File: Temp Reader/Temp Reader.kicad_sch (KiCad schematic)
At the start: 19 parts, among them U1 ESP32-WROOM-32, U2 BME280, U4 NRF24L01_Breakout, U5 AP62150WU

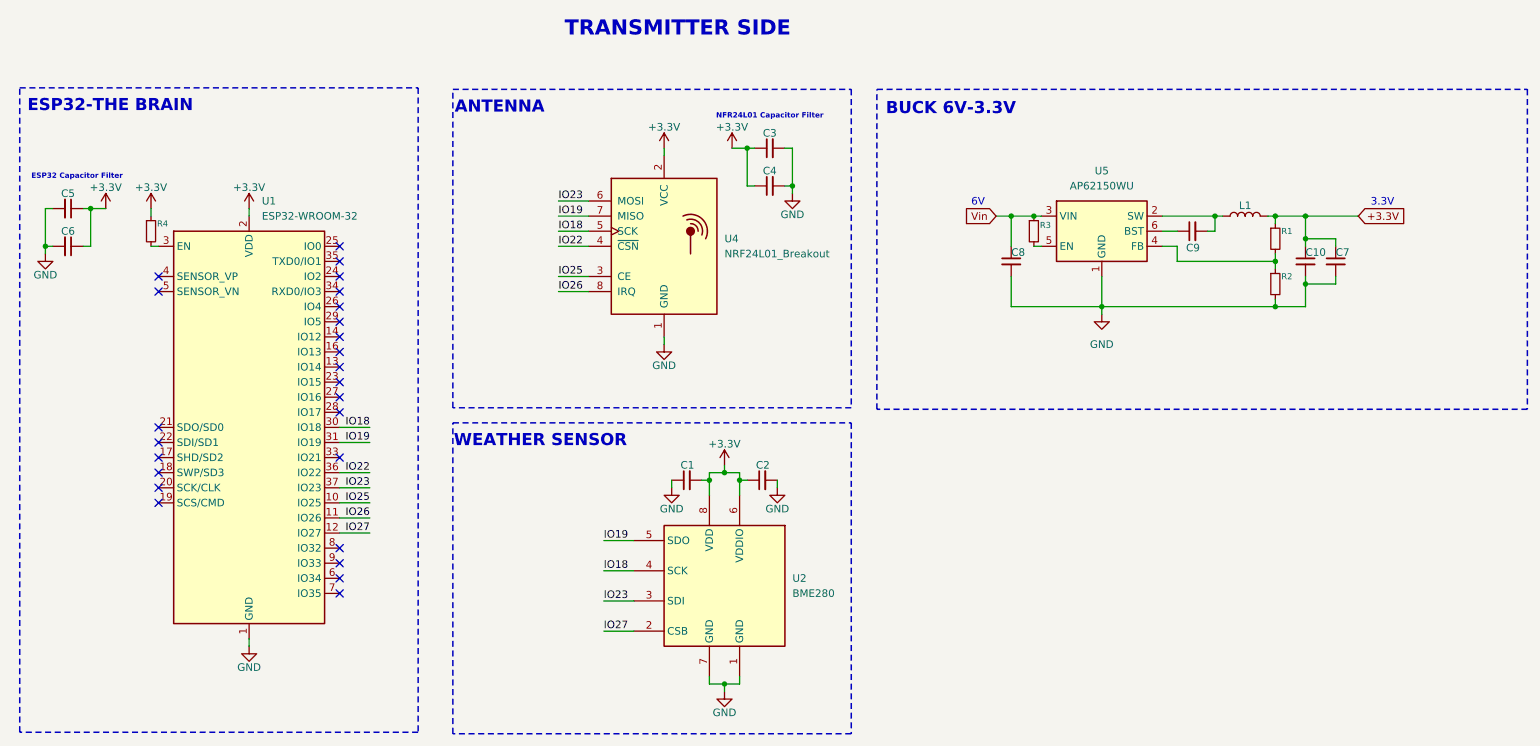
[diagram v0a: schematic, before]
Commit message: Final Schematic v 0.1.0
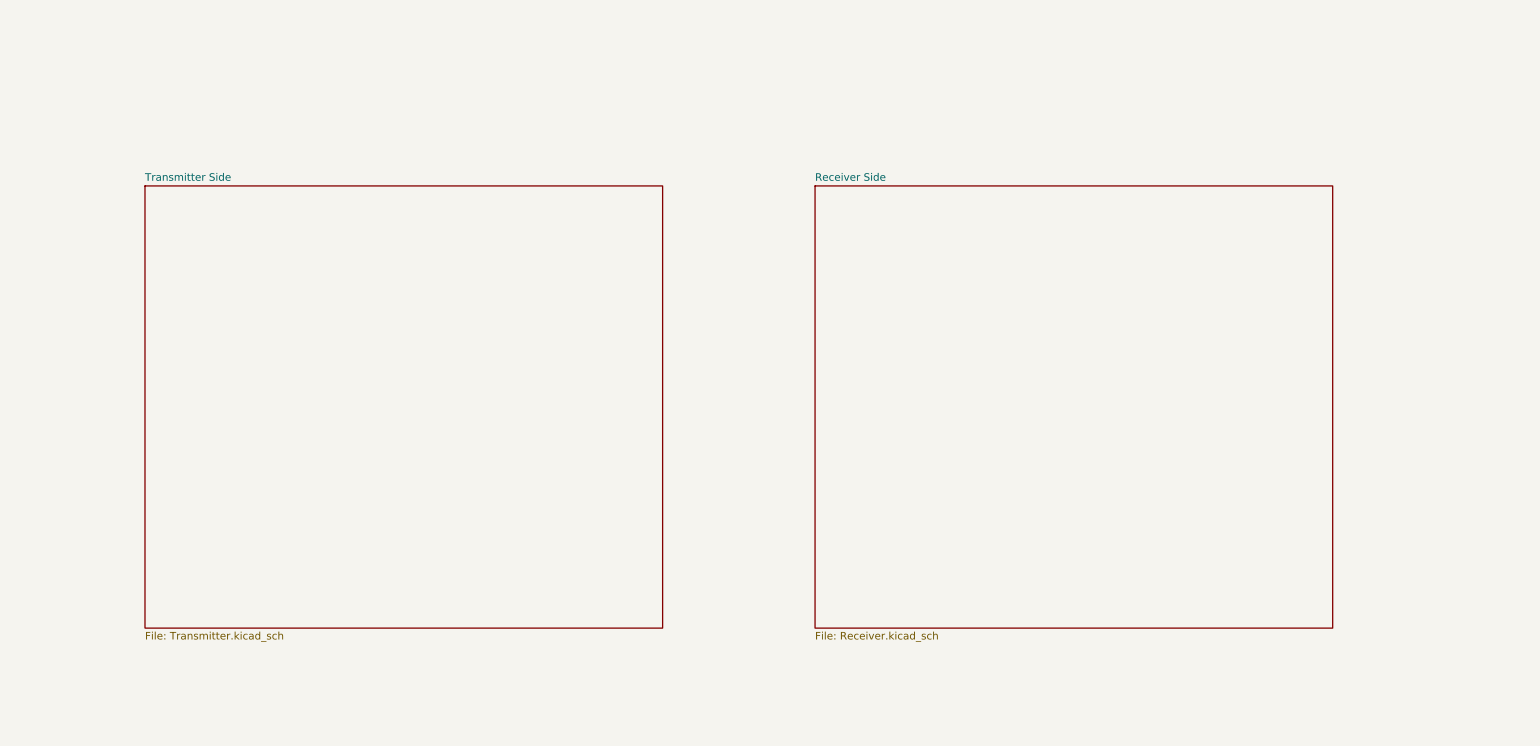
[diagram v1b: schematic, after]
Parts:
- removed C1, C2, C3, C5, C9: 100nF, Capacitor_SMD:C_0201_0603Metric, symbol Device:C_Small
- removed C10, C7, C8: 22uF, Capacitor_SMD:C_1206_3216Metric, symbol Device:C_Small
- removed C4, C6: 10uF, Capacitor_SMD:C_1206_3216Metric, symbol Device:C_Small
- removed L1: 2.2 uH, Inductor_SMD:L_Bourns-SRN4018, symbol Device:L
- removed R1: 31.25k, Resistor_SMD:R_0201_0603Metric, symbol Device:R_Small
- removed R2, R4: 10k, Resistor_SMD:R_0201_0603Metric, symbol Device:R_Small
- removed R3: 100k, Resistor_SMD:R_0201_0603Metric, symbol Device:R_Small
- removed U1: ESP32-WROOM-32, RF_Module:ESP32-WROOM-32, symbol RF_Module:ESP32-WROOM-32
- removed U2: BME280, Package_LGA:Bosch_LGA-8_2.5x2.5mm_P0.65mm_ClockwisePinNumbering, symbol Sensor:BME280
- removed U4: NRF24L01_Breakout, RF_Module:nRF24L01_Breakout, symbol RF:NRF24L01_Breakout
- removed U5: AP62150WU, Package_TO_SOT_SMD:TSOT-23-6, symbol Regulator_Switching:AP62150WU
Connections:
- no-connect marks 25 -> 0
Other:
- added sheet Receiver Side (Receiver.kicad_sch)
- added sheet Transmitter Side (Transmitter.kicad_sch)
- note removed: "3.3V"
- note removed: "6V"
- note removed: "ANTENNA"
- note removed: "BUCK 6V-3.3V"
- note removed: "ESP32 Capacitor Filter"
- note removed: "ESP32-THE BRAIN"
- note removed: "NFR24L01 Capacitor Filter"
- note removed: "TRANSMITTER SIDE"
- note removed: "WEATHER SENSOR"
